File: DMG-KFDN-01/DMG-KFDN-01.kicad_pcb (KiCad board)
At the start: 2 copper layers, 51.1 x 61.3 mm, 15 parts, among them U0 CartBus, U1 LH538MNP, U2 MBC3, U3 GM76C256CLLFW70, U4 BA6129AF, X1 Crystal

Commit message: KDFN -> KFDN (silkscr typo)
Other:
- board text added: "DMG-KFDN-01"
- board text removed: "DMG-KDFN-01"
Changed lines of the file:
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@@
     (effects (font (size 1.5 1.5) (thickness 0.3)) (justify mirror))
   )
-  (gr_text "DMG-KDFN-01" (at 154.94 70.5358) (layer "F.Mask")
+  (gr_text "DMG-KFDN-01" (at 154.94 70.5358) (layer "F.Mask")
     (effects (font (size 1.5 1.5) (thickness 0.3)))
   )

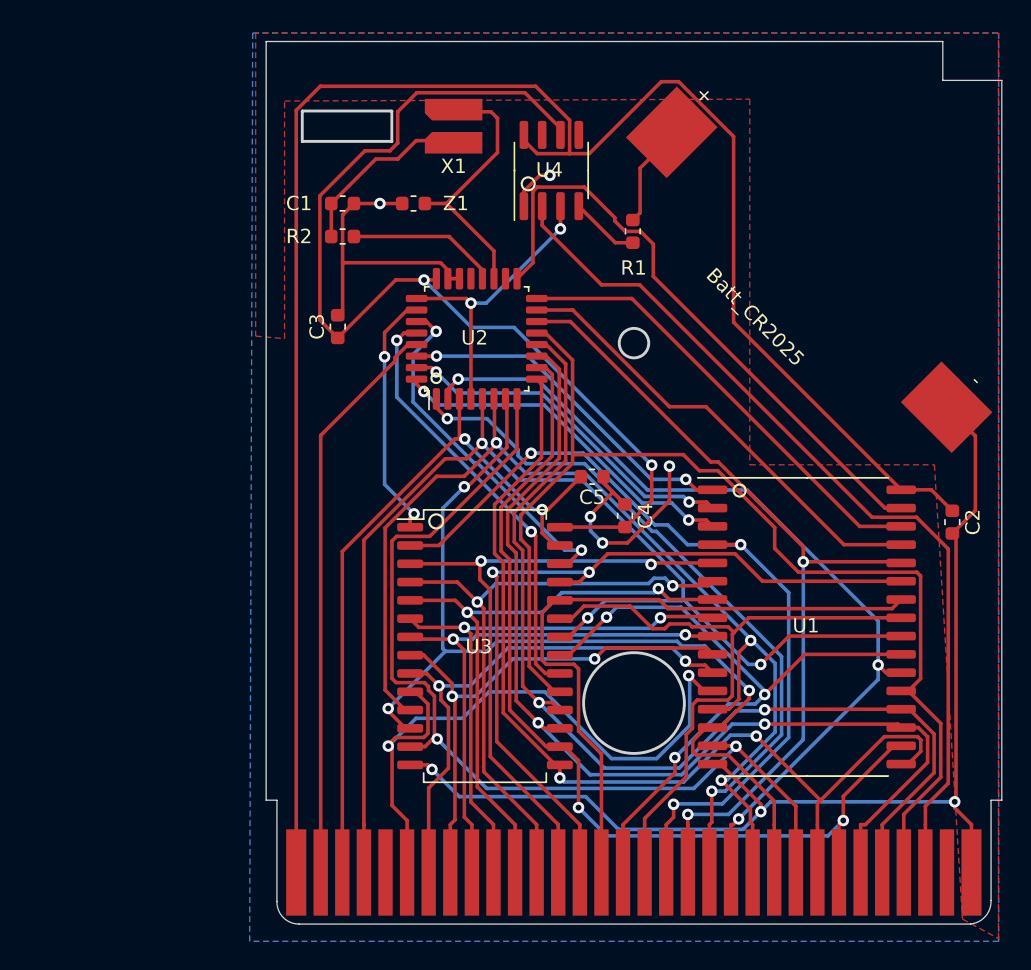
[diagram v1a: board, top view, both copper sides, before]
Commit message: Update DMG-KFDN-01
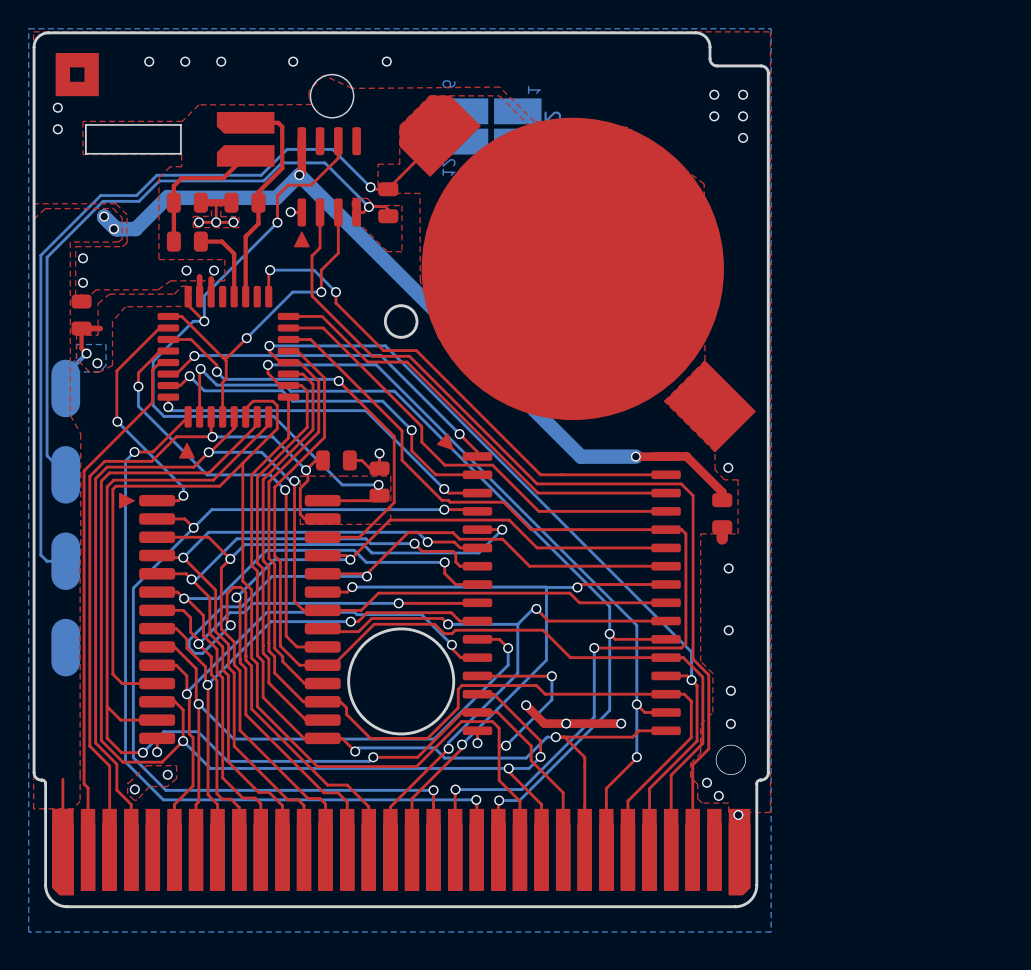
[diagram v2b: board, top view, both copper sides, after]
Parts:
- removed Batt_CR2025: Battery_Cell, NintendoFootprints:CR2025
- removed U0: CartBus, NintendoFootprints:CartBus
- added Batt CR2025: Battery_Cell, Custom:CR2025_Tabbed, F.Cu at (138.4, 84.5)
- added G***: LOGO, Custom:Nintendo-GBA-Logo, B.Cu at (142.1, 77.2)
- added J0: CartBus, HDR_Gameboy_Cartridges:GB_Cartridge_Front_Only, F.Cu at (126.5, 124.8)
- added TP1: RTC_VOUT, Custom:GameBoy_Testpoint, B.Cu at (103.2, 92.8)
- added TP2: VBatt, Custom:GameBoy_Testpoint, B.Cu at (103.2, 98.8)
- added TP3: BT+, Custom:GameBoy_Testpoint, B.Cu at (103.2, 104.8)
- added TP4: GND, Custom:GameBoy_Testpoint, B.Cu at (103.2, 110.8)
- added TP5: 3x3, HDR_Gameboy:3x3mm_Pad, F.Cu at (104.0, 71.0)
- added TP6: Date Indicator, HDR_Gameboy_Date_Indicators:12 December, B.Cu at (132.7, 74.6)
- C1, C2, C3, C4, C5: footprint Capacitor_SMD:C_0603_1608Metric -> Capacitor_SMD:C_0805_2012Metric
- R1, R2, Z1: footprint Resistor_SMD:R_0603_1608Metric -> Resistor_SMD:R_0805_2012Metric
- U3: footprint NintendoFootprints:GM76C256CLLFW70 -> Package_SO:SOIC-28W_7.5x17.9mm_P1.27mm
- moved C3 17.8 mm to (104.2, 87.7)
- moved C5 17.8 mm to (122.0, 97.8)
- moved U2 17.3 mm to (114.5, 90.6)
- moved C4 17.2 mm to (125.0, 99.3)
- moved R1 17.1 mm to (125.5, 79.9)
- moved U1 16.5 mm to (138.3, 107.1)
- moved C2 16.0 mm to (148.8, 101.5)
- moved U4 15.4 mm to (121.5, 78.1)
- moved X1 14.5 mm to (115.7, 75.5)
- moved U3 13.0 mm to (115.2, 108.8)
- moved Z1 11.7 mm to (115.6, 79.9)
- moved R2 10.8 mm to (111.6, 82.6)
- moved C1 10.8 mm to (111.6, 79.9)
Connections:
- net BattCS renamed \RST
- R1 pad 1: Net-(Batt_CR2025-Pad1) -> BT+
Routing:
- net GND: track 119.1 -> 23.3 mm, vias 8 -> 37
- net +5V: track 128.4 -> 64.5 mm, vias 0 -> 4
- net BT+: track 0.00 -> 56.5 mm, vias 0 -> 1
- net Batt: track 4.81 -> 44.9 mm, vias 0 -> 1
- net A9: track 46.7 -> 71.4 mm, vias 0 -> 2
- net D4: track 66.3 -> 83.0 mm, vias 2 -> 3
- net D0: track 76.5 -> 92.7 mm, vias 3 -> 2
- net Vout: track 72.1 -> 56.3 mm, vias 2 -> 5
- net D1: track 68.7 -> 82.0 mm
- net D6: track 72.8 -> 85.2 mm
- net D7: track 81.1 -> 69.7 mm
- net A13: track 59.4 -> 69.7 mm
- net D2: track 68.5 -> 77.2 mm
- net A1: track 37.0 -> 44.8 mm
- net A0: track 47.1 -> 39.7 mm
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- added copper zone on F.Cu, net +5V
- added copper zone on F.Cu, net BT+
- added copper zone on F.Cu, net Batt
- added copper zone on B.Cu, net Vout
- added copper zone on F.Cu, net Vout
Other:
- board size 51.1 x 61.3 mm -> 51 x 60.7 mm
- rule pad_to_mask_clearance: 0.0508 -> 0
- board text added: "1"
- board text added: "2022"
- board text added: "32"
- board text added: "C"
- board text added: "GND"
- board text added: "VDD"
- board text removed: "V1.0"

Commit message: Remove logos
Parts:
- removed G***: LOGO, Custom:Nintendo-GBA-Logo
